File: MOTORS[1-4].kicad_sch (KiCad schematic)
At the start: 13 parts, among them U22 ZX-SH1.0-8PWT

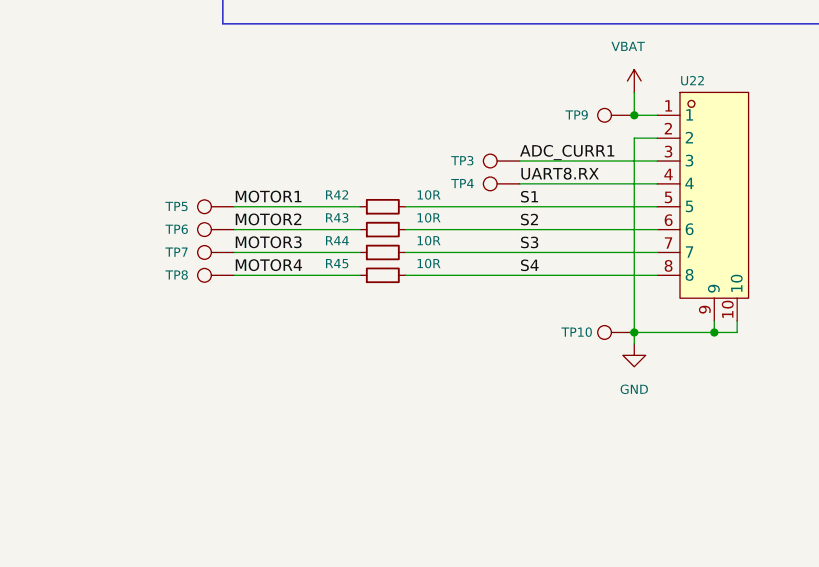
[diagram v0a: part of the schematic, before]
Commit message: power routing
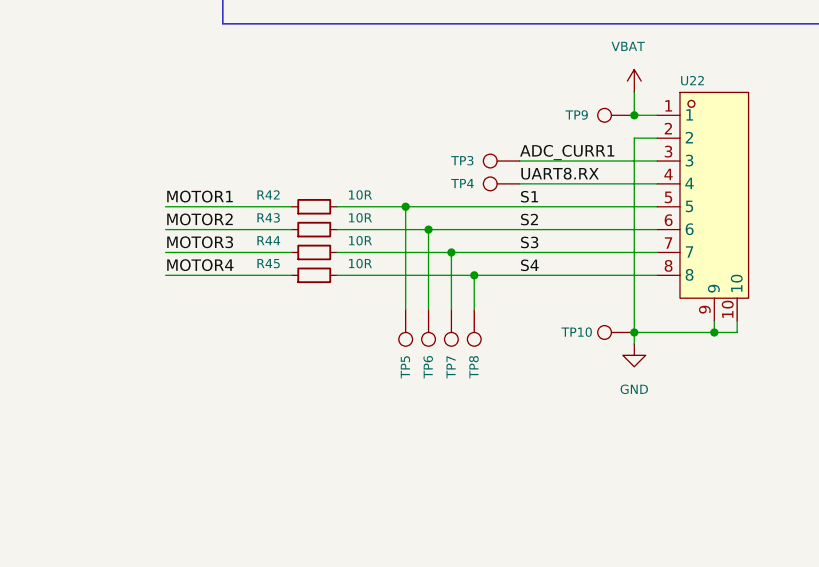
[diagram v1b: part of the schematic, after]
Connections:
- net MOTOR1: no longer TP5.1
- net MOTOR2: no longer TP6.1
- net MOTOR3: no longer TP7.1
- net MOTOR4: no longer TP8.1
- net S1: now also TP5.1
- net S2: now also TP6.1
- net S3: now also TP7.1
- net S4: now also TP8.1
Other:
- moved on the sheet: R42, R43, R44, R45
